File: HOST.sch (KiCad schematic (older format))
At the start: 8 parts

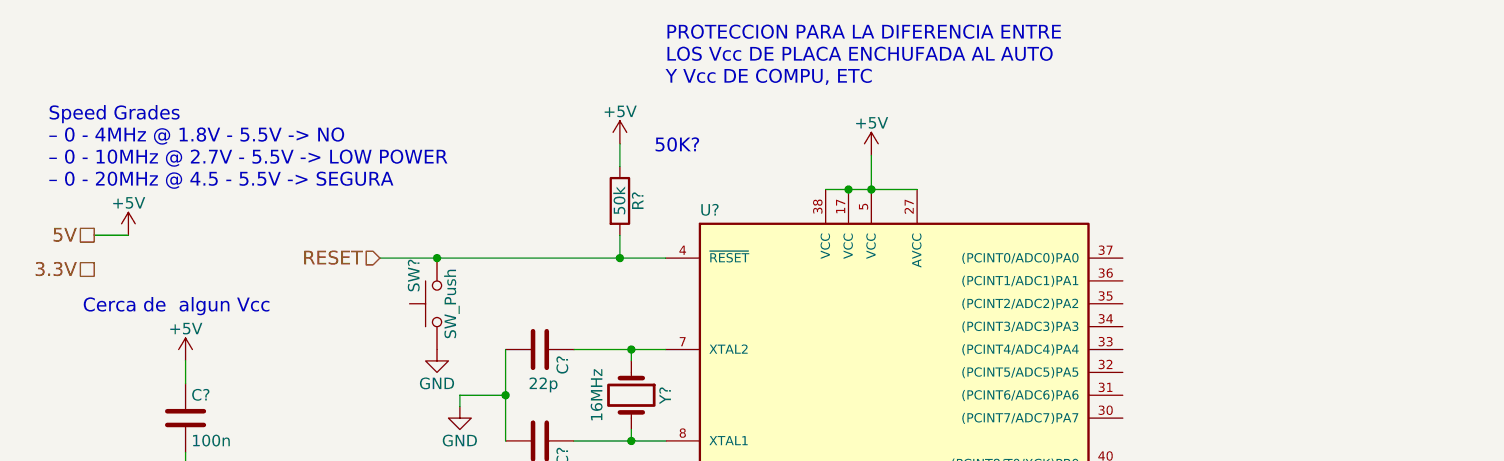
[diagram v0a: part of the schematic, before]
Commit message: ready for first rev
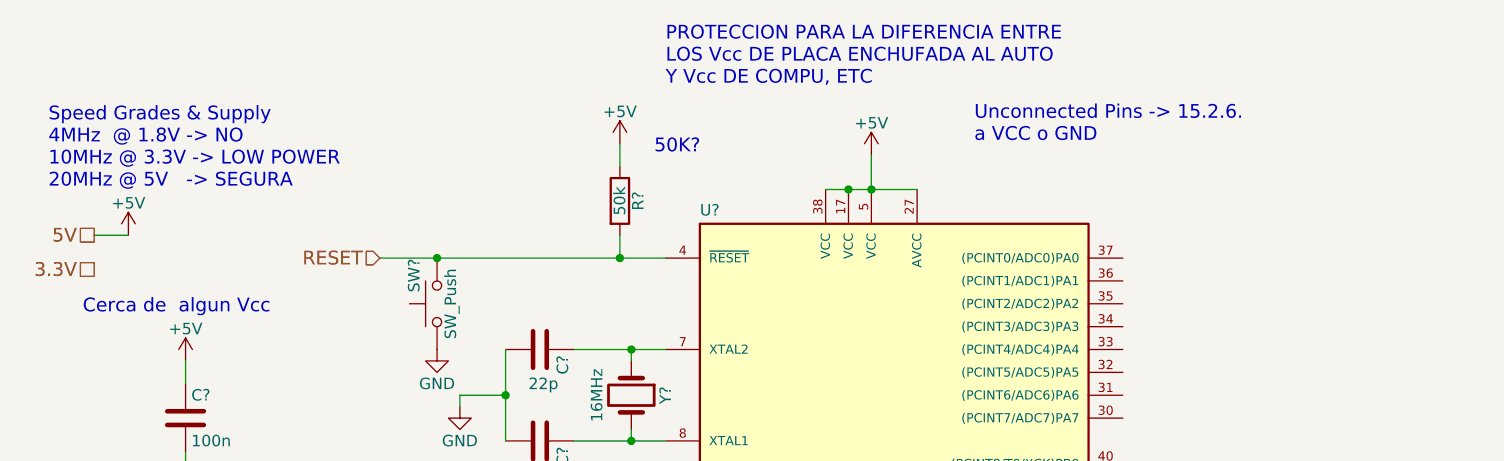
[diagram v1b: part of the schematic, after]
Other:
- note added: "Speed Grades & Supply\n4MHz @ 1.8V -> NO\n10MHz @ 3.3V -> LOW POWER\n20MHz @ 5V -> SEGURA"
- note added: "Unconnected Pins -> 15.2.6.\na VCC o GND"
- note removed: "Speed Grades\n– 0 - 4MHz @ 1.8V - 5.5V -> NO\n– 0 - 10MHz @ 2.7V - 5.5V -> LOW POWER\n– 0 - 20MHz @ 4.5 - 5.5V -> SEGURA"
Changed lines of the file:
@@
 3.3V
 Text Notes 1800 1450 0    60   ~ 0
-Speed Grades\n– 0 - 4MHz @ 1.8V - 5.5V -> NO\n– 0 - 10MHz @ 2.7V - 5.5V -> LOW POWER\n– 0 - 20MHz @ 4.5 - 5.5V -> SEGURA
+Speed Grades & Supply\n4MHz  @ 1.8V -> NO\n10MHz @ 3.3V -> LOW POWER\n20MHz @ 5V   -> SEGURA
 Text HLabel 7200 4450 2    60   Input ~ 0
 MASTER_BT_RX
@@
 	4300 1250 4300 1350
 Wire Wire Line
-	4300 1650 4300 1750
+	4300 1750 4300 1650
 Wire Wire Line
 	3250 1750 4500 1750
@@
 Wire Wire Line
 	6500 4950 7200 4950
+Text Notes 5850 1250 0    60   ~ 0
+Unconnected Pins -> 15.2.6.\na VCC o GND
 $EndSCHEMATC
